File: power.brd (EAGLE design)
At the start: 75.9 x 52.1 mm, 15 parts, among them Q1 MOSFET-NCHANNELSMD, Q2 MOSFET-NCHANNELSMD, U1 MCP73831, X1 Micro USB

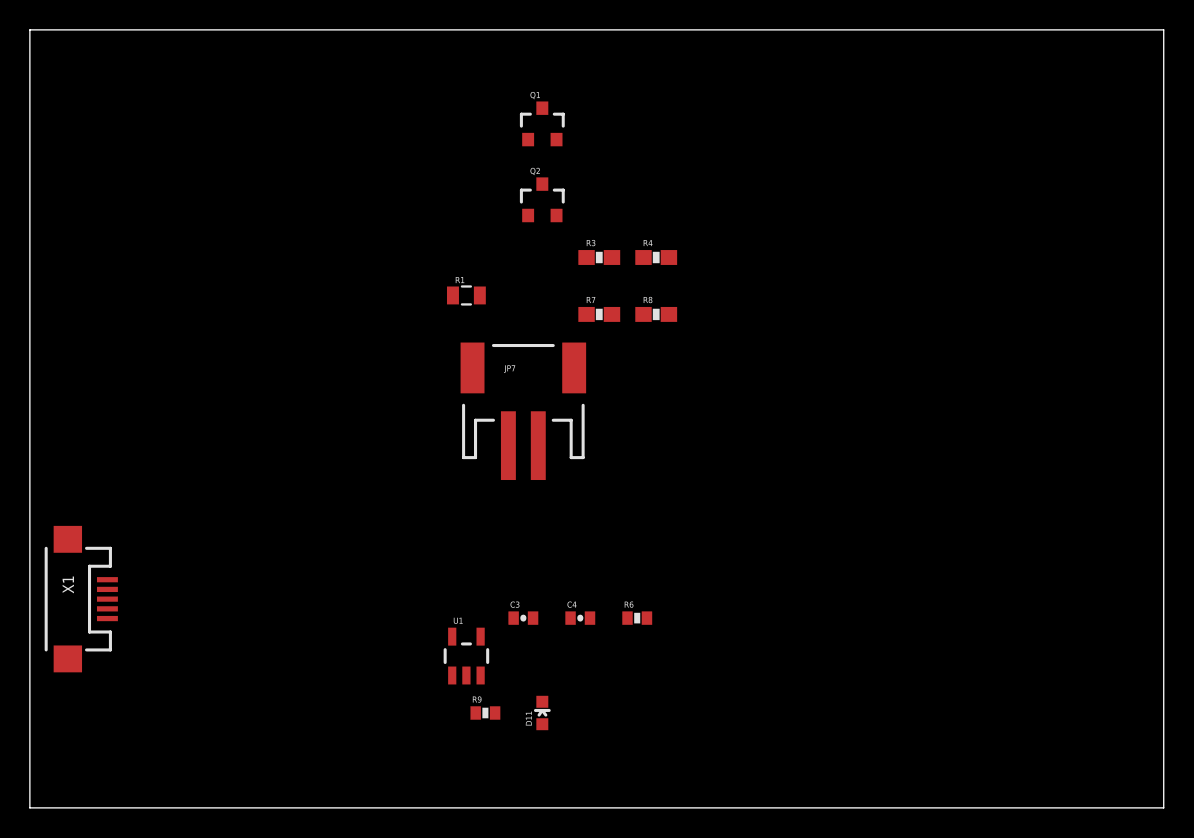
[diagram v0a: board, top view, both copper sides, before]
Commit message: Updating with changes
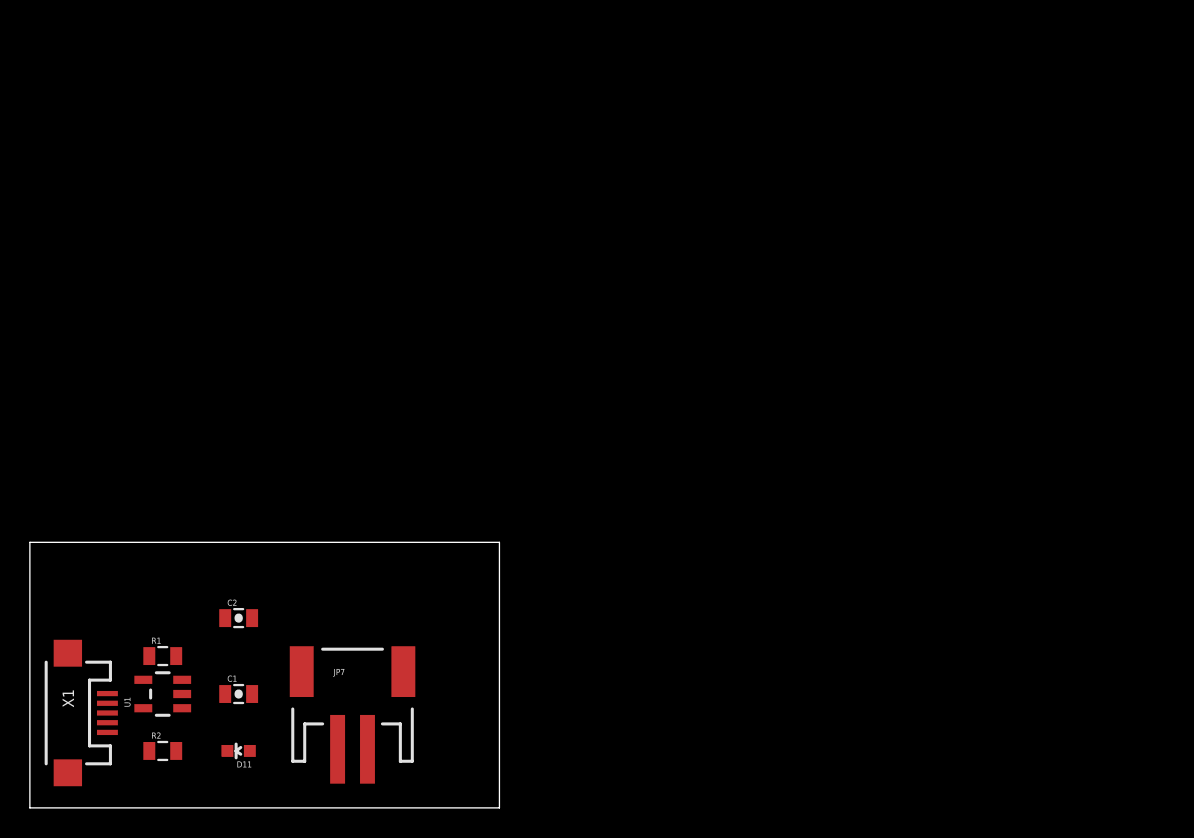
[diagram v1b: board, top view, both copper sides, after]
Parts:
- removed C3, C4: 4.7uF, SparkFun:0402-CAP
- removed Q1, Q2: MOSFET-NCHANNELSMD, SparkFun:SOT23-3
- removed R3, R4, R7, R8: 10K, SparkFun:0603-RES
- removed R6: 330, SparkFun:0402-RES
- removed R9: 2K, SparkFun:0402-RES
- added C1, C2: 4.7uF, SparkFun-Capacitors:0805-CAP
- added R2: 2k, SparkFun-Resistors:0805
- R1: value 10k -> 330
- moved R1 31.5 mm to (8.89, 10.2)
- moved JP7 23.3 mm to (21.6, 7.62)
- moved D11 20.5 mm to (14.0, 3.81), turned to 90 degrees
- moved U1 20.5 mm to (8.89, 7.62), turned to 90 degrees
- moved X1 7.62 mm to (2.54, 6.35)
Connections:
- removed net 3.3V: Q1.1, Q2.1, R3.1, R7.1
- removed net RTS: Q2.2, R7.2
- removed net RTS_5V: Q2.3, R8.2
- removed net TX: Q1.2, R3.2
- removed net TX_5V: Q1.3, R4.2
- net GND: now also C1.2, C2.2, R2.1; no longer C3.2, C4.2, R9.2
- net N$12: now also R1.2; no longer R6.1
- net PROG: now also R2.2; no longer R9.1
- net VCC: now also C2.1; no longer C4.1, R4.1, R8.1
- net VIN: now also C1.1, R1.1; no longer C3.1, R6.2
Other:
- board size 75.9 x 52.1 mm -> 31.4 x 17.8 mm
